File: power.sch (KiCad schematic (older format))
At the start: 52 parts, among them Q2 2N7002, Q3 2N7002, SW1 Pushbutton, U10 MCP73831, U11 INA213-SC70, U12 DRV8839, U13 DRV8839, U8 LT1965, U9 LTC2955DDB-1

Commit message: Change MCU to LQFP64 (instead of BGA)
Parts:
- added C34: 100uF, symbol C_Small
- added C36, C39: 10uF, symbol C_Small
- added R24: 3.3k, symbol R
- added R25: 2.05k, symbol R
- added U10: LT1965, MODULE, symbol LT1965
- D10, D11, D12, D13, D14, D15, D16, D8, D9: symbol LED -> LED-RESCUE-speedy
- Q2, Q3: symbol Q_NMOS_DGS -> Q_NMOS_DGS-RESCUE-speedy
- renumbered C36 to C31, C38 to C32, C35 to C33, C39 to C35, C40 to C37, C41 to C38, C37 to C40, C43 to C41, C44 to C43, C45 to C44, C46 to C45, C47 to C46, R20 to R19, R22 to R20, R23 to R21, R24 to R22, R25 to R23, R27 to R26, R28 to R27, R21 to R28, R26 to R29, R29 to R30, R30 to R31, R31 to R32, R32 to R33, R33 to R34, R34 to R35, U10 to U12, U12 to U13, U13 to U14, U9 to U8, U8 to U9
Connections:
- net labels added: SENSOR_EN, VCCA
- wire segments 155 -> 176
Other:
- note added: "Sensors power regulator (2.8V)\n"
- moved on the sheet: C31, C32, C33, C35, C37, C38, C40, C41, C42, C43, C44, C45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

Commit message: Netlist
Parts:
- C31, C32, C33, C34, C37, C40, C41, C42, C43, C44, F2, R19, R20, R21, R22, R23, R24, R25, R26, R27, R28, R29, R30, R31, R32, R33, R34, R35: footprint (none) -> _std:_0402
- C35, C36, C38, C39, C45, C46: footprint (none) -> _std:_0603
- CONN10, CONN11, CONN8, CONN9: footprint MODULE -> _connectors:_Solder_Pad1.27_2
- CONN7: footprint MODULE -> _connectors:_Pin2mm_2
- D10, D11, D12, D13, D14, D15, D16, D8, D9: footprint (none) -> LEDs:LED-0603
- Q2, Q3: footprint (none) -> _std:_SOT23-3
- SW1: footprint (none) -> _div:_PTS525SK15-SMT-Pushbutton
- U10, U9: footprint MODULE -> Housings_DFN_QFN:DFN-8-1EP_3x3mm_Pitch0.5mm
- U11: footprint (none) -> _std:SC70
- U12: footprint (none) -> _std:_TSOT23-5
- U13, U14, U8: footprint (none) -> Housings_DFN_QFN:DFN-10-1EP_2x3mm_Pitch0.5mm

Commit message: Remove CAN interface
(not useful enough, takes too much place)
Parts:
- U13, U14: footprint Housings_DFN_QFN:DFN-10-1EP_2x3mm_Pitch0.5mm -> _div:TI-DRV8839_PWSON-N12
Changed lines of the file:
@@
 F 0 "U13" H 8650 1900 59  0000 C CNN
 F 1 "DRV8839" H 8300 1900 59  0000 C CNN
-F 2 "Housings_DFN_QFN:DFN-10-1EP_2x3mm_Pitch0.5mm" H 8350 1700 39  0001 C CNN
+F 2 "_div:TI-DRV8839_PWSON-N12" H 8350 1700 39  0001 C CNN
 F 3 "" H 8350 1700 39  0000 C CNN
 	1    8400 1450
@@
 F 0 "U14" H 8650 3200 59  0000 C CNN
 F 1 "DRV8839" H 8300 3200 59  0000 C CNN
-F 2 "Housings_DFN_QFN:DFN-10-1EP_2x3mm_Pitch0.5mm" H 8350 3000 39  0001 C CNN
+F 2 "_div:TI-DRV8839_PWSON-N12" H 8350 3000 39  0001 C CNN
 F 3 "" H 8350 3000 39  0000 C CNN
 	1    8400 2750

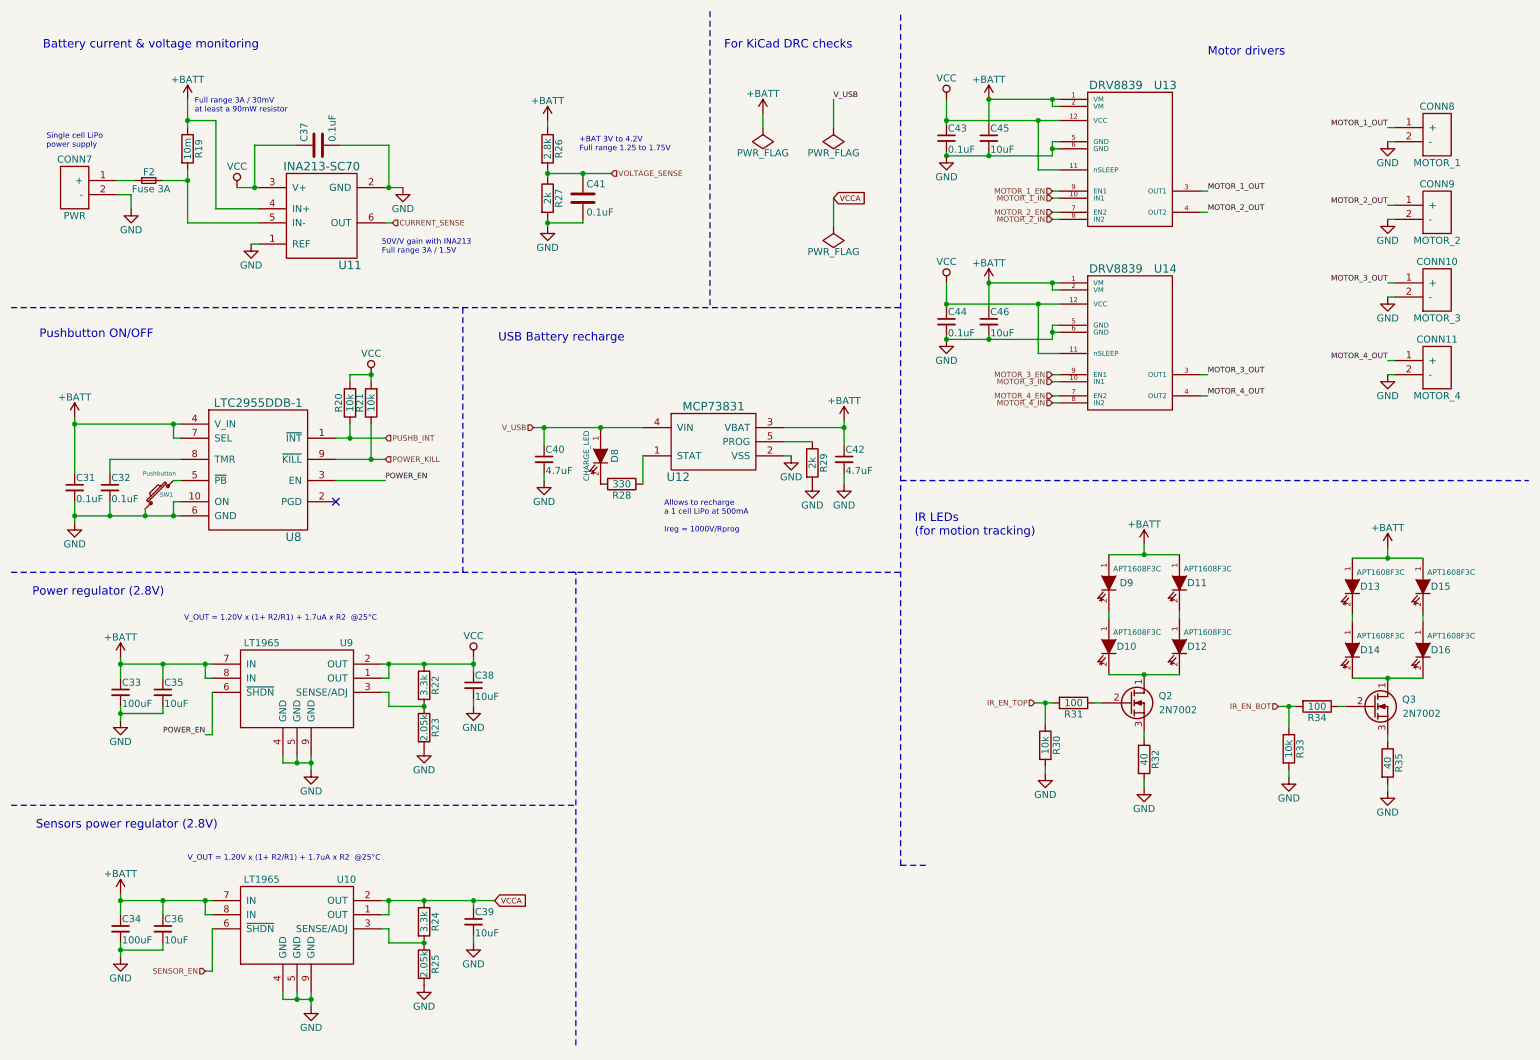
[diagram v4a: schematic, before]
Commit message: Remove SD card
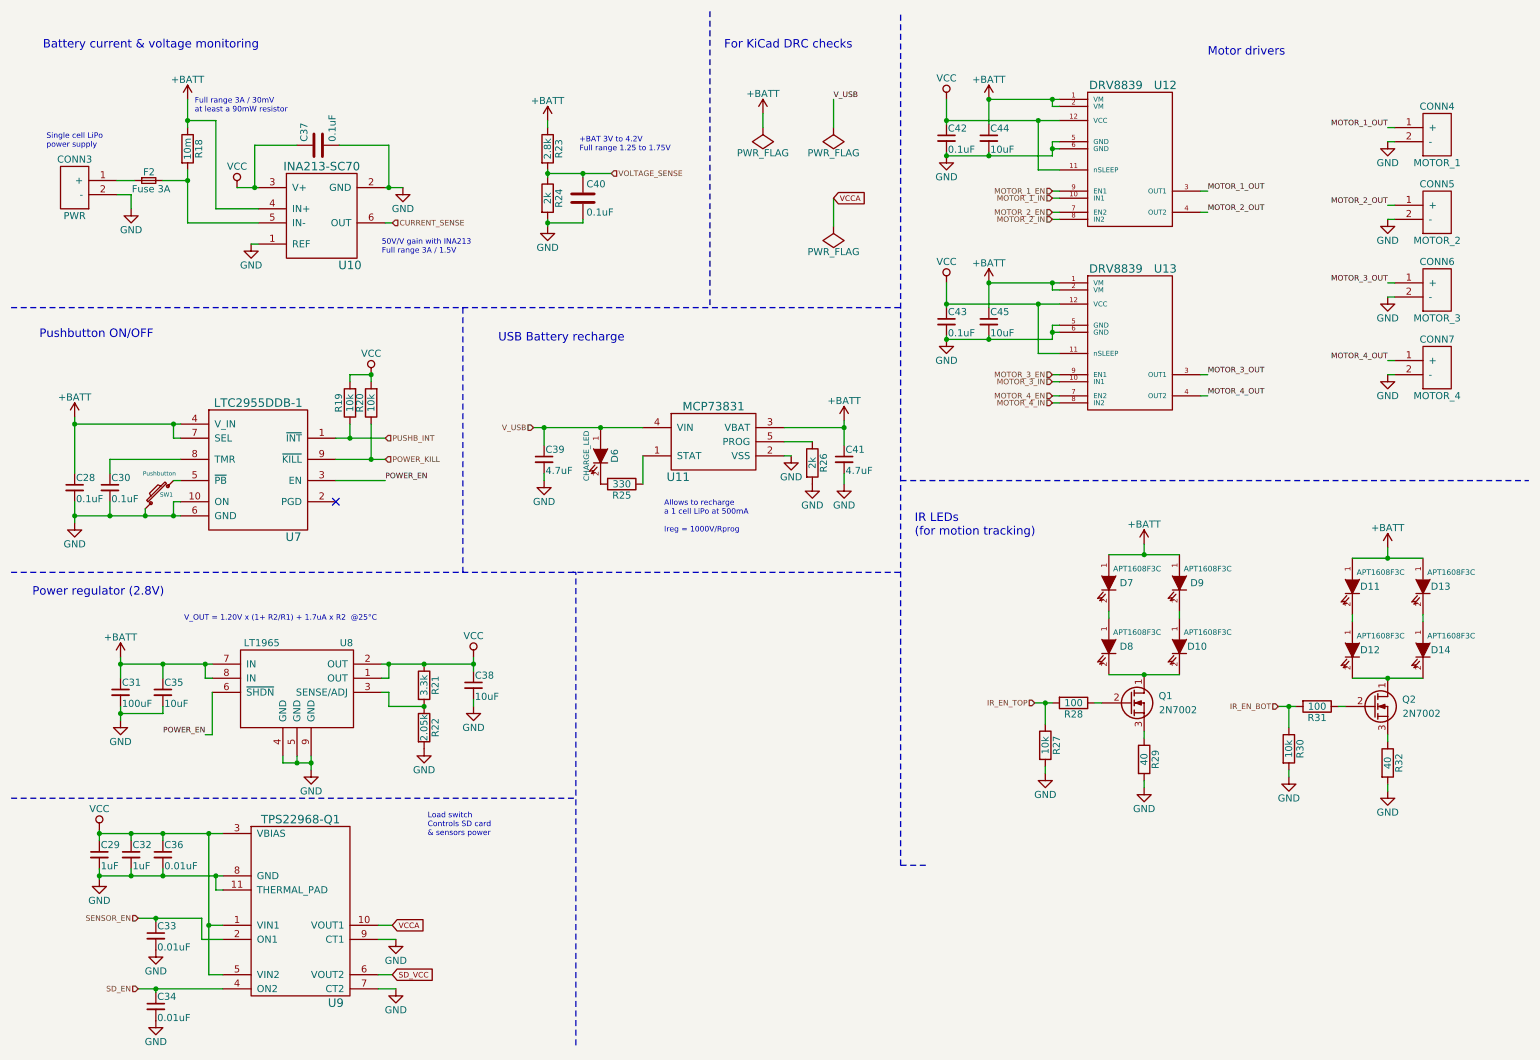
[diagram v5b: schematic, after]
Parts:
- removed C39: 10uF, _std:_0603, symbol C_Small
- removed R24: 3.3k, _std:_0402, symbol R
- removed R25: 2.05k, _std:_0402, symbol R
- removed U10: LT1965, Housings_DFN_QFN:DFN-8-1EP_3x3mm_Pitch0.5mm, symbol LT1965
- added C29, C32: 1uF, _std:_0402, symbol C_Small
- added C33: 0.01uF, _std:_0402, symbol C_Small
- added U9: TPS22968-Q1, _std:WSON10, symbol TPS22968-Q1
- C31: renamed from C33; footprint _std:_0402 -> _std:_0603
- C34: value 100uF -> 0.01uF
- C36: value 10uF -> 0.01uF; footprint _std:_0603 -> _std:_0402
- renumbered C31 to C28, C32 to C30, C40 to C39, C41 to C40, C42 to C41, C43 to C42, C44 to C43, C45 to C44, C46 to C45, CONN7 to CONN3, CONN8 to CONN4, CONN9 to CONN5, CONN10 to CONN6, CONN11 to CONN7, D12 to D10, D13 to D11, D14 to D12, D15 to D13, D16 to D14, D8 to D6, D9 to D7, D10 to D8, D11 to D9, Q2 to Q1, Q3 to Q2, R19 to R18, R20 to R19, R21 to R20, R22 to R21, R23 to R22, R26 to R23, R27 to R24, R28 to R25, R29 to R26, R30 to R27, R31 to R28, R32 to R29, R33 to R30, R34 to R31, R35 to R32, U11 to U10, U12 to U11, U13 to U12, U14 to U13, U8 to U7, U9 to U8
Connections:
- net +BATT: no longer C34.1, C36.1
- net GND: now also C29.2, C32.2, C33.2, U9.11 (THERMAL_PAD), U9.7 (CT2), U9.8 (GND), U9.9 (CT1)
- net SENSOR_EN: now also C33.1, U9.2 (ON1)
- net VCC: now also C36.1, C29.1, C32.1, U9.1 (VIN1), U9.3 (VBIAS), U9.5 (VIN2)
- net VCCA: now also U9.10 (VOUT1)
- new net SD_EN: C34.1, U9.4 (ON2)
- new net SD_VCC: U9.6 (VOUT2)
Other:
- note added: "Load switch\nControls SD card \n& sensors power"
- note removed: "Sensors power regulator (2.8V)\n"

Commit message: Revert "Remove SD card"
This reverts commit 4a1918bee256f93cb8d66746410e6c192988175c.
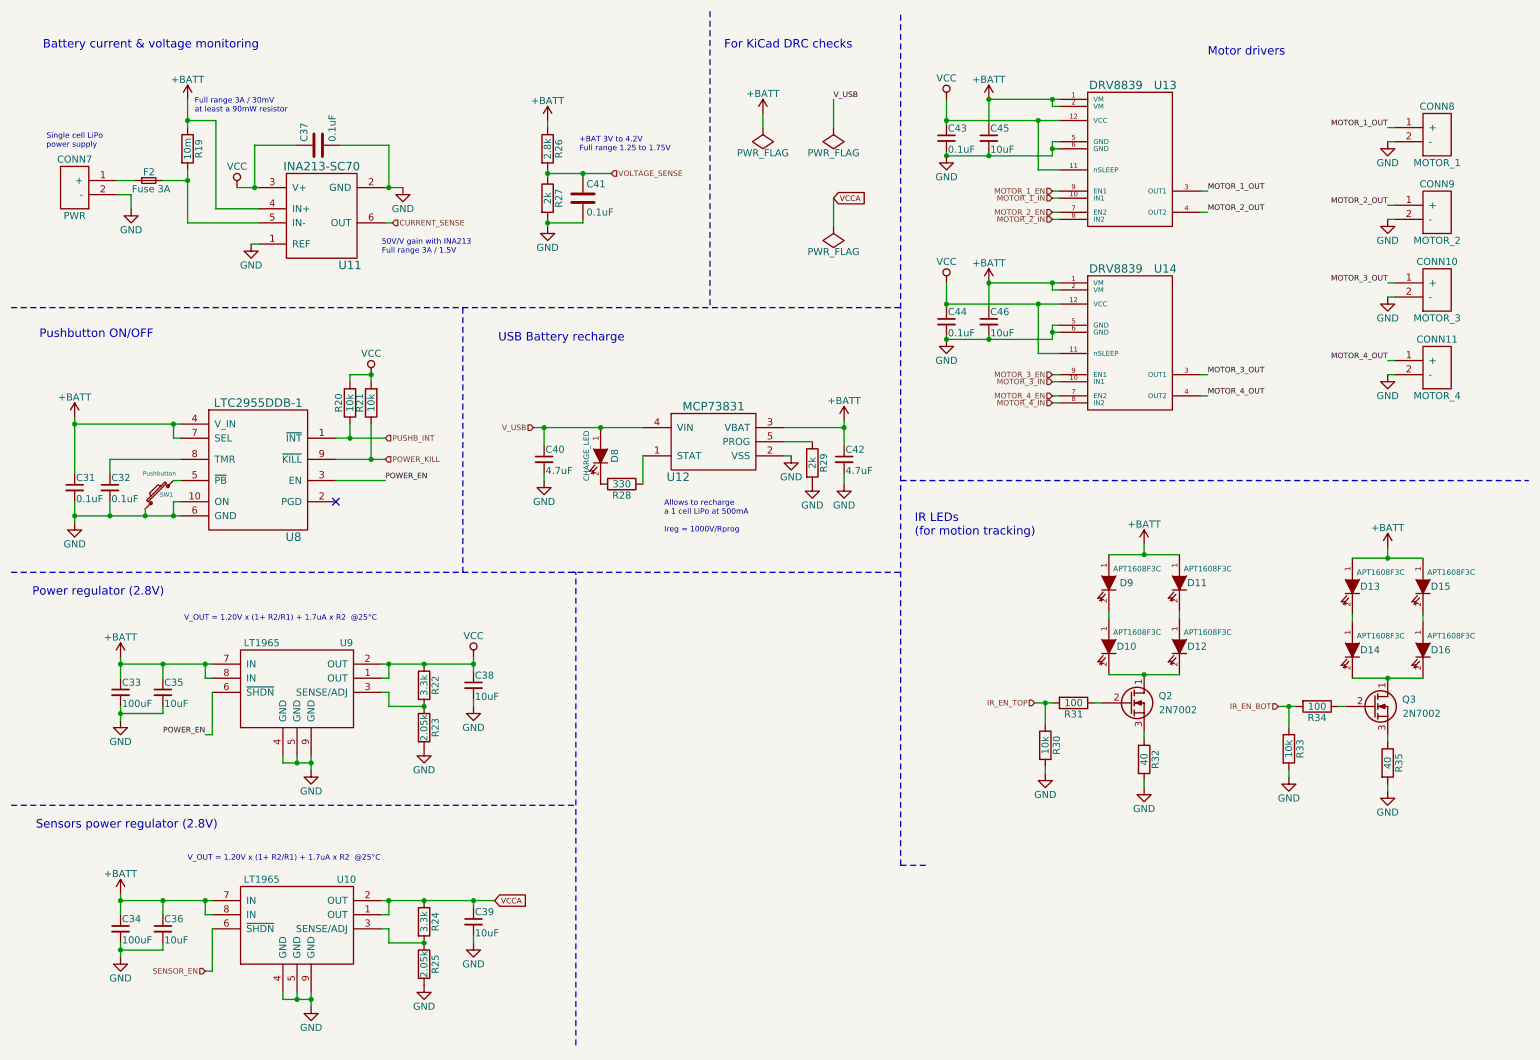
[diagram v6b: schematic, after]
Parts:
- removed C29, C32: 1uF, _std:_0402, symbol C_Small
- removed C33: 0.01uF, _std:_0402, symbol C_Small
- removed U9: TPS22968-Q1, _std:WSON10, symbol TPS22968-Q1
- added C39: 10uF, _std:_0603, symbol C_Small
- added R24: 3.3k, _std:_0402, symbol R
- added R25: 2.05k, _std:_0402, symbol R
- added U10: LT1965, Housings_DFN_QFN:DFN-8-1EP_3x3mm_Pitch0.5mm, symbol LT1965
- C33: renamed from C31; footprint _std:_0603 -> _std:_0402
- C34: value 0.01uF -> 100uF
- C36: value 0.01uF -> 10uF; footprint _std:_0402 -> _std:_0603
- renumbered C28 to C31, C30 to C32, C39 to C40, C40 to C41, C41 to C42, C42 to C43, C43 to C44, C44 to C45, C45 to C46, CONN6 to CONN10, CONN7 to CONN11, CONN3 to CONN7, CONN4 to CONN8, CONN5 to CONN9, D8 to D10, D9 to D11, D10 to D12, D11 to D13, D12 to D14, D13 to D15, D14 to D16, D6 to D8, D7 to D9, Q1 to Q2, Q2 to Q3, R18 to R19, R19 to R20, R20 to R21, R21 to R22, R22 to R23, R23 to R26, R24 to R27, R25 to R28, R26 to R29, R27 to R30, R28 to R31, R29 to R32, R30 to R33, R31 to R34, R32 to R35, U10 to U11, U11 to U12, U12 to U13, U13 to U14, U7 to U8, U8 to U9
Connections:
- net SD_EN is gone; now on net +BATT: C34.1
- net +BATT: now also C36.1, U10.7 (IN), U10.8 (IN)
- net GND: now also C39.2, R25.2, U10.4 (GND), U10.5 (GND), U10.9 (GND)
- net SENSOR_EN: now also U10.6 (~SHDN)
- net VCC: no longer C36.1
- net VCCA: now also C39.1, R24.1, U10.1 (OUT), U10.2 (OUT)
- new net: R24.2, R25.1, U10.3 (SENSE/ADJ)
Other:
- note added: "Sensors power regulator (2.8V)\n"
- note removed: "Load switch\nControls SD card \n& sensors power"
